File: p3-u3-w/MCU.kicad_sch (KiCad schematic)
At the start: 27 parts, among them J1 SWD_pin, SW1 SW_SPST, U2 STM32WB55RGVx, X1 NX2016SA-32MHZ-EXS00A-CS06654, Y1 32k768

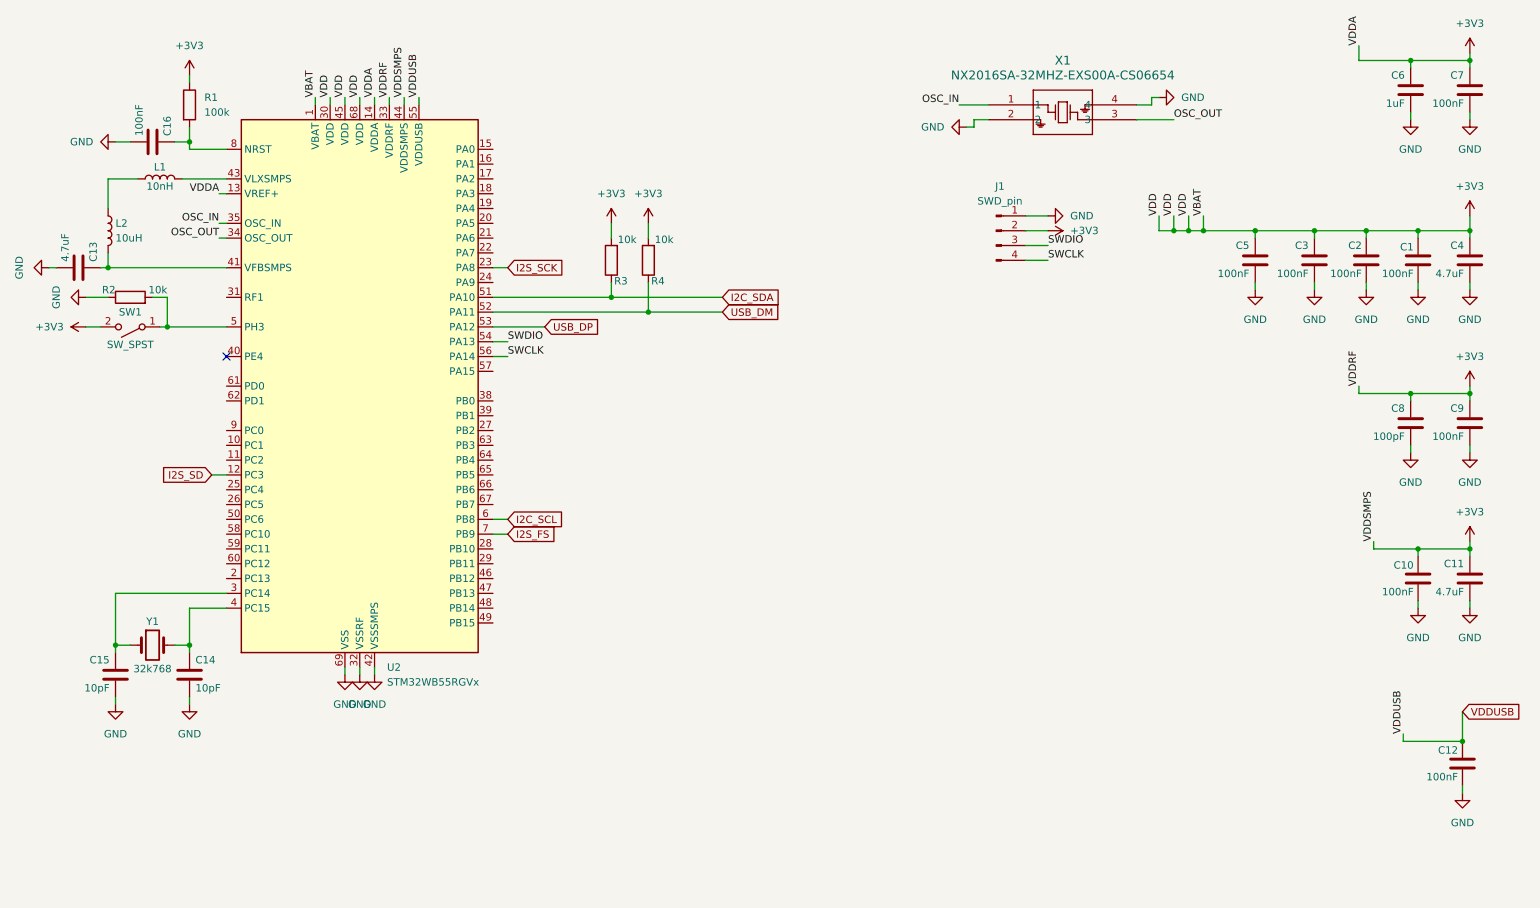
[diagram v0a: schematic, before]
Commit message: added in power side and mostly finished schematics :)
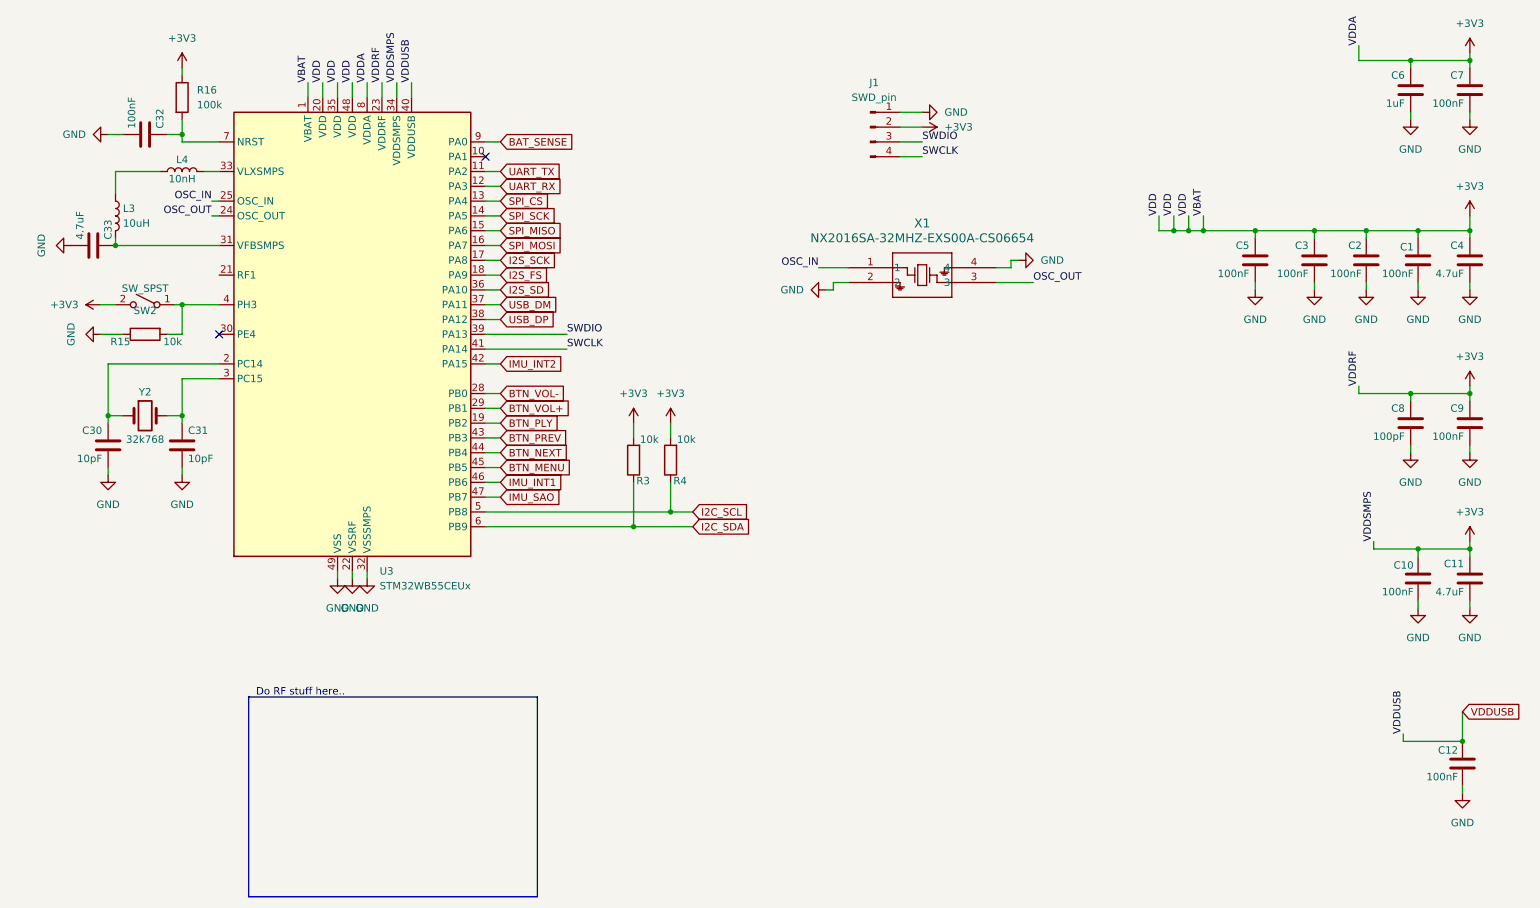
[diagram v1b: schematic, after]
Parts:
- removed C13: 4.7uF, symbol Device:C
- removed C14, C15: 10pF, symbol Device:C
- removed C16: 100nF, symbol Device:C
- removed L1: 10nH, symbol Device:L
- removed L2: 10uH, symbol Device:L
- removed R1: 100k, symbol Device:R
- removed R2: 10k, symbol Device:R
- removed SW1: SW_SPST, symbol Switch:SW_SPST
- removed U2: STM32WB55RGVx, Package_DFN_QFN:QFN-68-1EP_8x8mm_P0.4mm_EP6.4x6.4mm, symbol MCU_ST_STM32WB:STM32WB55RGVx
- removed Y1: 32k768, symbol Device:Crystal
- added C30, C31: 10pF, symbol Device:C
- added C32: 100nF, symbol Device:C
- added C33: 4.7uF, symbol Device:C
- added L3: 10uH, symbol Device:L
- added L4: 10nH, symbol Device:L
- added R15: 10k, symbol Device:R
- added R16: 100k, symbol Device:R
- added SW2: SW_SPST, symbol Switch:SW_SPST
- added U3: STM32WB55CEUx, Package_DFN_QFN:QFN-48-1EP_7x7mm_P0.5mm_EP5.6x5.6mm, symbol MCU_ST_STM32WB:STM32WB55CEUx
- added Y2: 32k768, symbol Device:Crystal
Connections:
- net +3V3: now also R16.1, SW2.2 (B), U3.1 (VBAT), U3.20 (VDD), U3.23 (VDDRF), U3.34 (VDDSMPS), U3.35 (VDD), U3.48 (VDD), U3.8 (VDDA)
- net GND: now also C30.1, C31.1, C32.1, C33.1, R15.1, U3.22 (VSSRF), U3.32 (VSSSMPS), U3.49 (VSS)
- net I2C_SCL: now also R4.1, U3.5 (PB8)
- net I2C_SDA: now also U3.6 (PB9)
- net I2S_FS: now also U3.18 (PA9)
- net I2S_SCK: now also U3.17 (PA8)
- net I2S_SD: now also U3.36 (PA10)
- net OSC_IN: now also U3.25 (OSC_IN)
- net OSC_OUT: now also U3.24 (OSC_OUT)
- net SWCLK: now also U3.41 (PA14)
- net SWDIO: now also U3.39 (PA13)
- net USB_DM: now also U3.37 (PA11); no longer R4.1
- net USB_DP: now also U3.38 (PA12)
- net VDDUSB: now also U3.40 (VDDUSB)
- new net: R15.2, SW2.1 (A), U3.4 (PH3)
- new net: C33.2, L3.2, U3.31 (VFBSMPS)
- new net: C31.2, U3.3 (PC15), Y2.2
- new net: C32.2, R16.2, U3.7 (NRST)
- new net: C30.2, U3.2 (PC14), Y2.1
- new net: L4.2, U3.33 (VLXSMPS)
- new net: L3.1, L4.1
- new net BAT_SENSE: U3.9 (PA0)
- new net BTN_MENU: U3.45 (PB5)
- new net BTN_NEXT: U3.44 (PB4)
- new net BTN_PLY: U3.19 (PB2)
- new net BTN_PREV: U3.43 (PB3)
- new net BTN_VOL+: U3.29 (PB1)
- new net BTN_VOL-: U3.28 (PB0)
- new net IMU_INT1: U3.46 (PB6)
- new net IMU_INT2: U3.42 (PA15)
- new net IMU_SAO: U3.47 (PB7)
- new net SPI_CS: U3.13 (PA4)
- new net SPI_MISO: U3.15 (PA6)
- new net SPI_MOSI: U3.16 (PA7)
- new net SPI_SCK: U3.14 (PA5)
- new net UART_RX: U3.12 (PA3)
- new net UART_TX: U3.11 (PA2)
- no-connect marks 1 -> 2
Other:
- note added: "Do RF stuff here.."
- moved on the sheet: J1, R3, R4, X1
